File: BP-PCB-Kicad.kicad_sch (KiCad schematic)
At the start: 23 parts, among them J1 Conn_02x25_Odd_Even, J10 A3C-4DA-2DSA_71_, J11 Conn_02x25_Odd_Even, J12 A3C-4DA-2DSA_71_, J15 Conn_02x25_Odd_Even, J16 DF14-15P-1.25H52, J17 DF14-30P-1.25H_35_, J18 DF14-15P-1.25H52, J19 DF14-15P-1.25H52, J20 A3C-50DA-2DSA_71_, J21 A3C-50DA-2DSA_71_, J22 A3C-50DA-2DSA_71_, J23 A3C-50DA-2DSA_71_, J24 A3C-50DA-2DSA_71_, J25 Molex 55460-0272, J26 Molex 55460-0272, J27 Molex 55460-0272, J28 Conn_01x20, J29 Conn_01x20, J5 Conn_02x25_Odd_Even, J7 A3C-4DA-2DSA_71_, J8 Conn_02x25_Odd_Even, J9 A3C-4DA-2DSA_71_

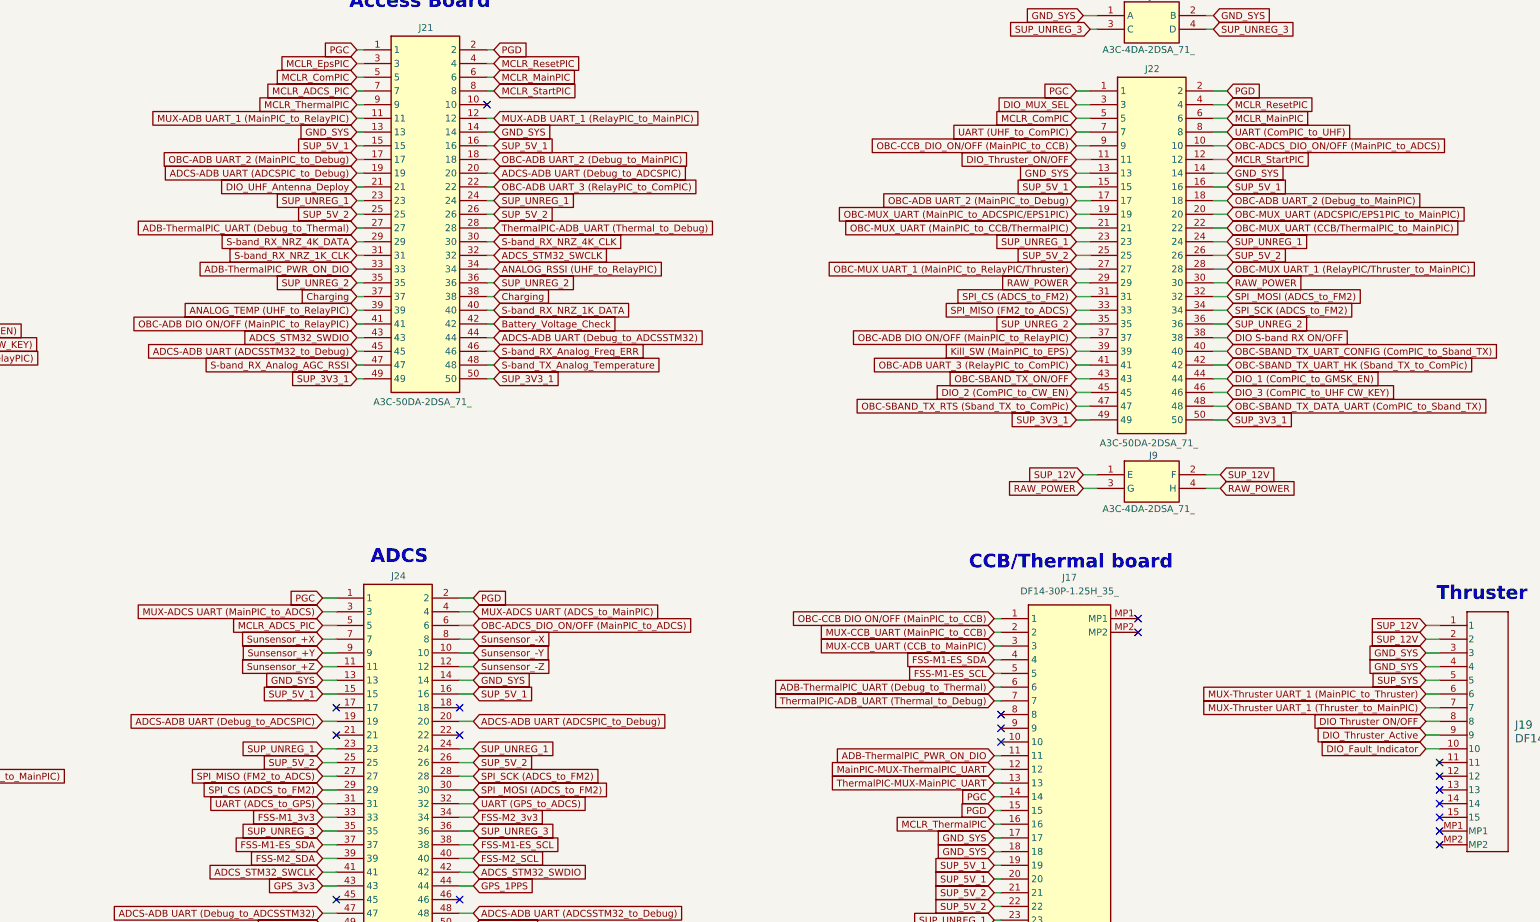
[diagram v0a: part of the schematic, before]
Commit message: Adjusted to libraries
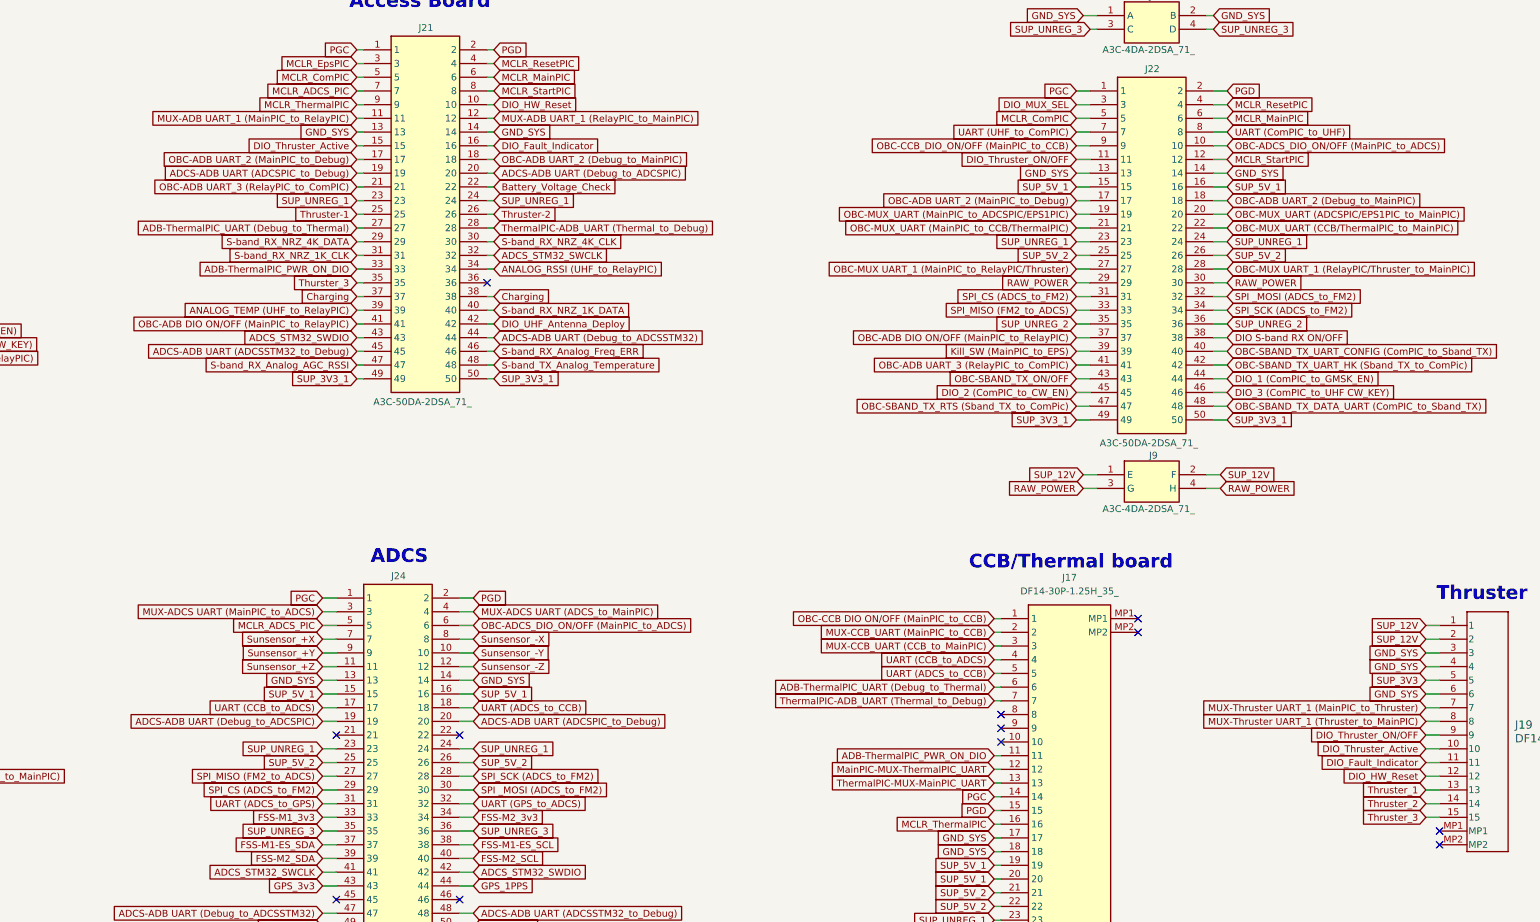
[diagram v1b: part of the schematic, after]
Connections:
- net DIO Thruster ON/OFF is gone; now on net MUX-Thruster UART_1 (Thruster_to_MainPIC): J19.8
- net Battery_Voltage_Check: now also J21.22; no longer J21.42
- net DIO_Fault_Indicator: now also J19.11, J21.16; no longer J19.10
- net DIO_Thruster_Active: now also J19.10, J21.15; no longer J19.9
- net DIO_Thruster_ON/OFF: now also J19.9
- net DIO_UHF_Antenna_Deploy: now also J21.42; no longer J21.21
- net FSS-M1-ES_SCL: no longer J17.5
- net FSS-M1-ES_SDA: no longer J17.4
- net GND_SYS: now also J19.6
- net MUX-Thruster UART_1 (MainPIC_to_Thruster): now also J19.7; no longer J19.6
- net MUX-Thruster UART_1 (Thruster_to_MainPIC): no longer J19.7
- net OBC-ADB UART_3 (RelayPIC_to_ComPIC): now also J21.21; no longer J21.22
- net SUP_5V_1: no longer J21.15, J21.16
- net SUP_5V_2: no longer J21.25, J21.26
- net SUP_UNREG_2: no longer J21.35, J21.36
- net DIO_HW_Reset: now reaches J21.10
- net DIO_HW_Reset: now also J19.12
- net UART (CCB_to_ADCS): now reaches J24.17
- net UART (CCB_to_ADCS): now also J17.4
- net UART (ADCS_to_CCB): now reaches J24.18
- net UART (ADCS_to_CCB): now also J17.5
- net Thruster_1: now reaches J19.13
- net Thruster_2: now reaches J19.14
- net Thruster_3: now reaches J19.15
- net SUP_SYS renamed SUP_3V3
- new net Thruster-1: J21.25
- new net Thruster-2: J21.26
- new net Thurster_3: J21.35
- no-connect marks 76 -> 69
